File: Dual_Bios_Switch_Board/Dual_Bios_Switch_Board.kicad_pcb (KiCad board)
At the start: 2 copper layers, 19.1 x 16.8 mm, 6 parts, among them J1 Conn_02x04_Counter_Clockwise, SW1 SW_DPDT_x2, U1 SOIC-8, U2 SOIC-8

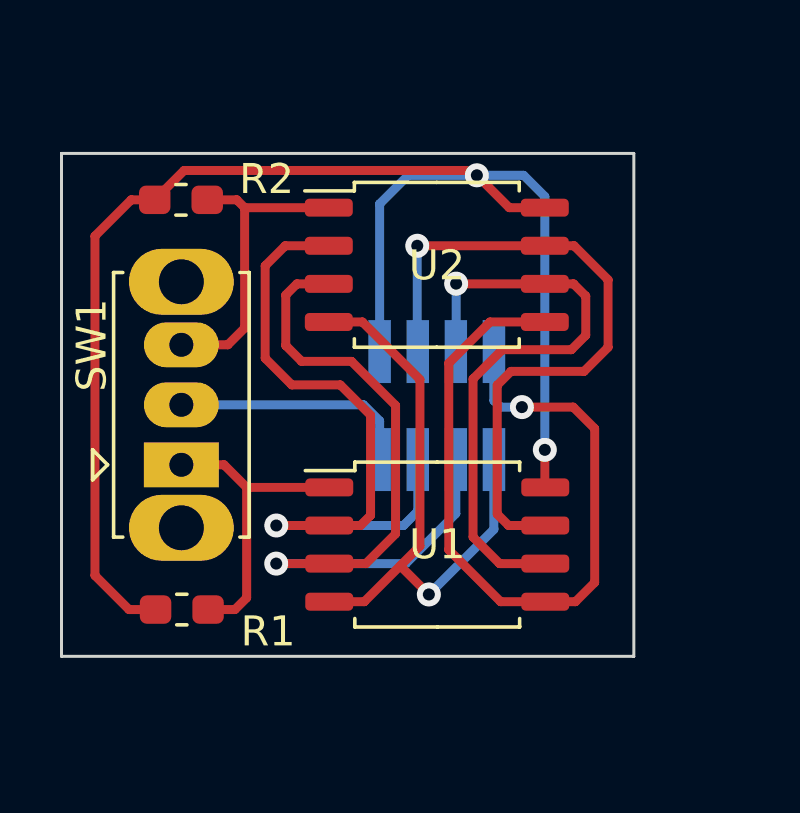
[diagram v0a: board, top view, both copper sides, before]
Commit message: fix details issues
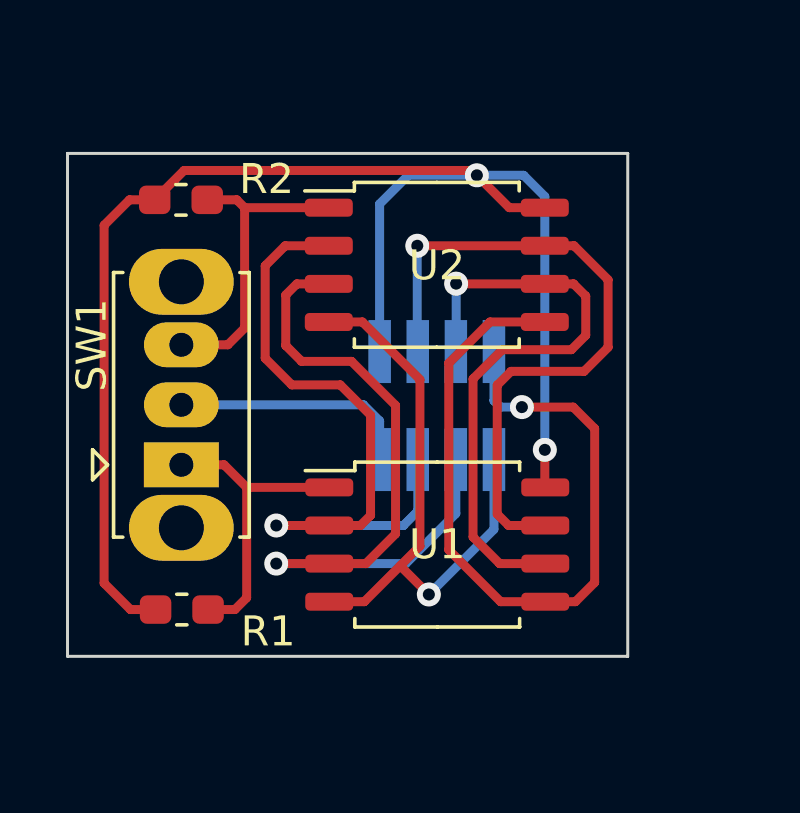
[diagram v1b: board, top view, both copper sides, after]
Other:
- board size 19.1 x 16.8 mm -> 18.7 x 16.8 mm
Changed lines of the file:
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@@
     )
   )
-  (gr_line (start 187.67552 147.828) (end 206.75346 147.828) (layer Edge.Cuts) (width 0.1))
-  (gr_line (start 187.67552 131.064) (end 206.75346 131.064) (layer Edge.Cuts) (width 0.1))
-  (gr_line (start 206.75346 131.064) (end 206.75346 147.828) (layer Edge.Cuts) (width 0.1))
-  (gr_line (start 187.67552 147.828) (end 187.67552 131.064) (layer Edge.Cuts) (width 0.1))
-  (segment (start 190.78324 132.61086) (end 189.99962 132.61086) (width 0.3) (layer F.Cu) (net 1))
-  (segment (start 189.99962 132.61086) (end 188.79058 133.8199) (width 0.3) (layer F.Cu) (net 1))
-  (segment (start 188.79058 133.8199) (end 188.79058 145.13306) (width 0.3) (layer F.Cu) (net 1))
-  (segment (start 189.92596 146.26844) (end 190.81118 146.26844) (width 0.3) (layer F.Cu) (net 1))
-  (segment (start 188.79058 145.13306) (end 189.92596 146.26844) (width 0.3) (layer F.Cu) (net 1))
+  (gr_line (start 187.87618 147.828) (end 206.55026 147.828) (layer Edge.Cuts) (width 0.1))
+  (gr_line (start 187.87618 131.064) (end 206.55026 131.064) (layer Edge.Cuts) (width 0.1))
+  (gr_line (start 206.55026 131.064) (end 206.55026 147.828) (layer Edge.Cuts) (width 0.1))
+  (gr_line (start 187.87618 147.828) (end 187.87618 131.064) (layer Edge.Cuts) (width 0.1))
   (segment (start 203.78502 132.87248) (end 202.60056 132.87248) (width 0.3) (layer F.Cu) (net 1))
   (segment (start 202.60056 132.87248) (end 201.52106 131.79298) (width 0.3) (layer F.Cu) (net 1))
@@
   (segment (start 203.78674 142.1833) (end 203.80026 142.19682) (width 0.3) (layer F.Cu) (net 1))
   (segment (start 203.78674 140.9446) (end 203.78674 142.1833) (width 0.3) (layer F.Cu) (net 1))
+  (segment (start 190.78324 132.61086) (end 189.94374 132.61086) (width 0.3) (layer F.Cu) (net 1))
+  (segment (start 189.94374 132.61086) (end 189.09538 133.45922) (width 0.3) (layer F.Cu) (net 1))
+  (segment (start 190.81118 146.26844) (end 189.97422 146.26844) (width 0.3) (layer F.Cu) (net 1))
+  (segment (start 189.09538 145.3896) (end 189.09538 133.45922) (width 0.3) (layer F.Cu) (net 1))
+  (segment (start 189.97422 146.26844) (end 189.09538 145.3896) (width 0.3) (layer F.Cu) (net 1))
   (segment (start 203.78502 134.14248) (end 204.7621 134.14248) (width 0.3) (layer F.Cu) (net 2))
   (segment (start 204.7621 134.14248) (end 205.89494 135.27532) (width 0.3) (layer F.Cu) (net 2))

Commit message: bump version to 2.0
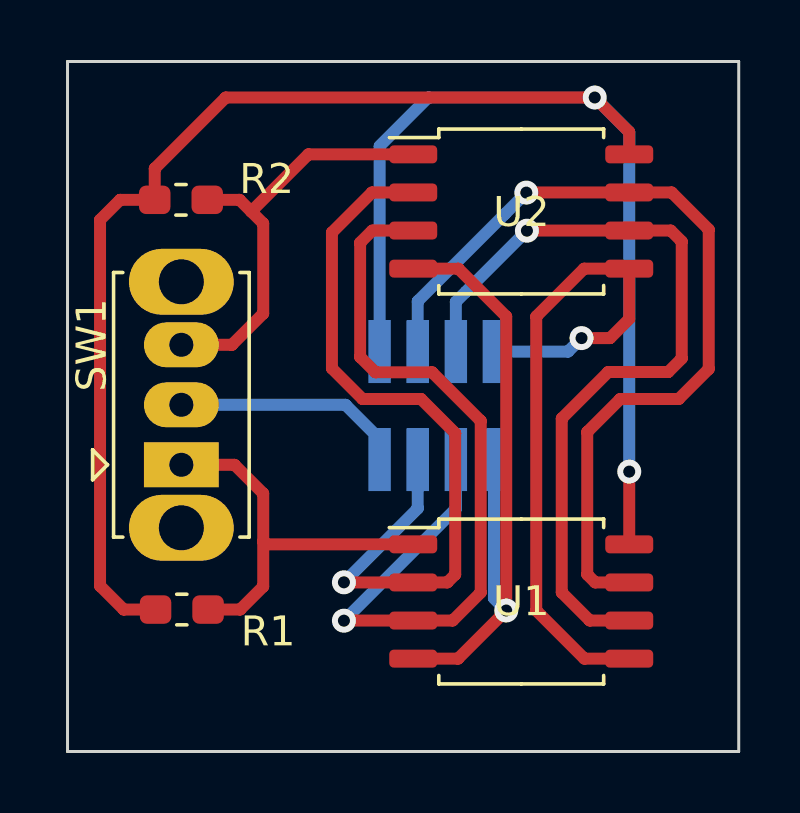
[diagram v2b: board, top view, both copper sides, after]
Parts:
- moved U1 3.38 mm to (203.0, 146.0)
- moved U2 3.33 mm to (203.0, 133.0)
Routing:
- net VCC: track 50.8 -> 65.6 mm
- net CLK: track 20.5 -> 27.5 mm
- net HOLD: track 22.9 -> 29.2 mm
- net CS2: track 10.5 -> 14.5 mm
- net DO: track 23.0 -> 26.4 mm
- net WP: track 24.9 -> 28.2 mm
- net CS1: track 10.4 -> 13.4 mm
- net GND: track 19.9 -> 22.5 mm
- net DI: track 26.3 -> 24.0 mm
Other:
- board size 18.7 x 16.8 mm -> 22.4 x 23 mm
- net class Default removed
